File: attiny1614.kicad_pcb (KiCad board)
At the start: 2 copper layers, 14.7 x 18.8 mm, 12 parts, among them J1 Conn_01x07, J2 Conn_01x07, J3 Conn_01x02, J4 UPDI, U1 AP7381-50SA, U2 ATtiny1614-SS

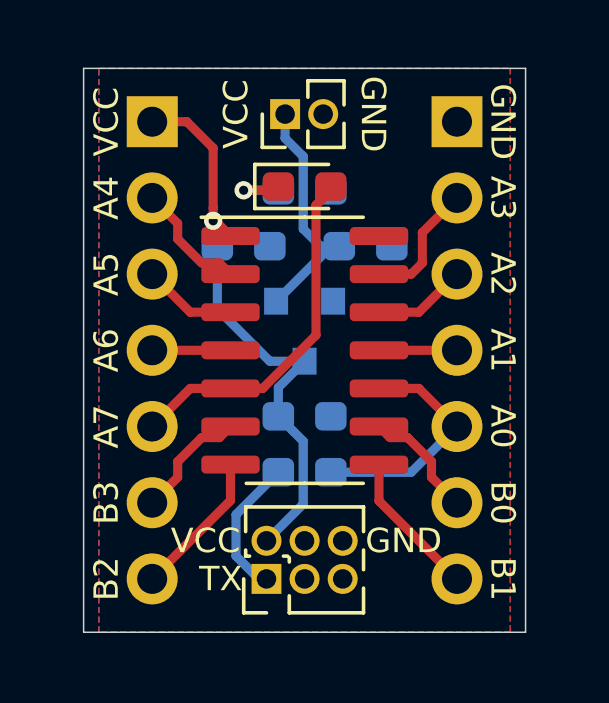
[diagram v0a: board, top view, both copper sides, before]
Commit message: gerbers and layout
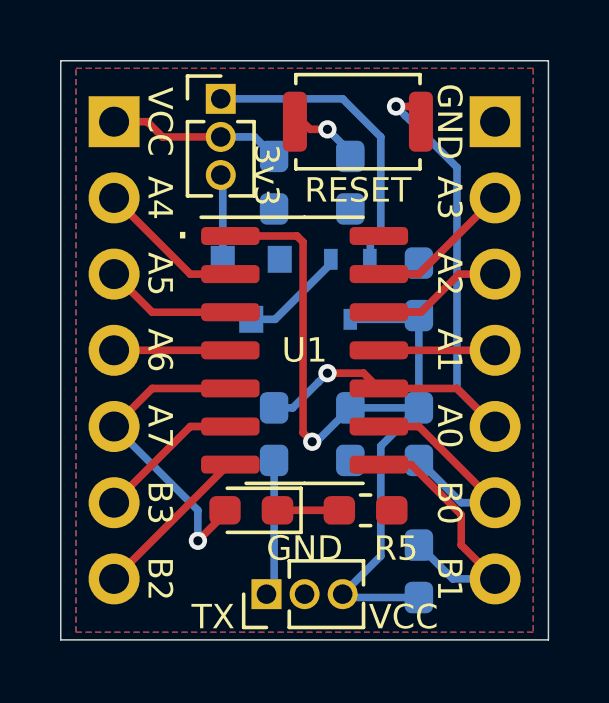
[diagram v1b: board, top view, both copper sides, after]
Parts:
- removed J4: UPDI, Connector_PinHeader_1.27mm:PinHeader_2x03_P1.27mm_Vertical
- added D2: BAT54CW, Package_TO_SOT_SMD:SOT-323_SC-70, B.Cu at (132.1, 87.9)
- added JP1: VCC Select, Connector_PinHeader_1.27mm:PinHeader_1x03_P1.27mm_Vertical, F.Cu at (127.8, 81.5)
- added R3: 10K, Resistor_SMD:R_0603_1608Metric_Pad1.05x0.95mm_HandSolder, B.Cu at (134.4, 97.3)
- added R4: 4.7K, Resistor_SMD:R_0603_1608Metric_Pad1.05x0.95mm_HandSolder, B.Cu at (129.5, 92.7)
- added R5: 2.2K, Resistor_SMD:R_0603_1608Metric_Pad1.05x0.95mm_HandSolder, F.Cu at (132.6, 95.2)
- added SW1: Reset, Button_Switch_SMD:SW_Push_SPST_NO_Alps_SKRK, F.Cu at (132.3, 82.3)
- J1: value Conn_01x07 -> UPDI; footprint Connector_PinHeader_2.54mm:PinHeader_1x07_P2.54mm_Vertical -> Connector_PinHeader_1.27mm:PinHeader_1x03_P1.27mm_Vertical; moved to F.Cu
- J3: value Conn_01x02 -> Conn_01x07; footprint Connector_PinHeader_1.27mm:PinHeader_1x02_P1.27mm_Vertical -> Connector_PinHeader_2.54mm:PinHeader_1x07_P2.54mm_Vertical; moved to B.Cu
- R1: value 4.7K -> 100R
- R2: value 4.7K -> 10K
- U1: value AP7381-50SA -> ATtiny1614-SS; footprint Package_TO_SOT_SMD:SOT-23 -> Package_SO:SOIC-14_3.9x8.7mm_P1.27mm; moved to F.Cu
- U2: value ATtiny1614-SS -> AP7381-33SA; footprint Package_SO:SOIC-14_3.9x8.7mm_P1.27mm -> Package_TO_SOT_SMD:SOT-23; moved to B.Cu
- moved J1 16.2 mm to (129.3, 98.0), turned to 90 degrees
- moved J2 11.4 mm to (124.2, 82.3)
- moved D1 10.9 mm to (128.8, 95.2), turned to 180 degrees
- moved R1 9.77 mm to (132.1, 84.3), turned to 270 degrees
- moved R2 8.98 mm to (134.4, 92.7), turned to 90 degrees
- moved C3 7.20 mm to (132.1, 92.7), turned to 270 degrees
- moved J3 7.00 mm to (136.9, 82.3), turned to 180 degrees
- moved C2 5.69 mm to (134.4, 87.9), turned to 90 degrees
- moved C1 3.71 mm to (129.5, 84.3), turned to 270 degrees
- moved U2 2.70 mm to (128.8, 87.9), turned to 270 degrees
- moved U1 0.63 mm to (130.6, 89.9), turned to 0 degrees
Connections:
- D1 pad 1: Net-(D1-Pad1) -> Net-(D2-Pad1)
- J1 pad 1: VCC -> /TX
- J1 pad 2: /PA4 -> GND
- J1 pad 3: /PA5 -> VCC
- J2 pad 1: GND -> /V_in
- J2 pad 2: /PA3 -> /PA4
- J2 pad 3: /PA2 -> /PA5
- J2 pad 4: /PA1 -> /PA6
- J2 pad 5: /PA0 -> /PA7
- J2 pad 6: /PB0 -> /RXD
- J2 pad 7: /PB1 -> /TXD
- J3 pad 1: /V_in -> GND
- J3 pad 2: GND -> /SCK
- R1 pad 1: /TX -> Net-(R1-Pad1)
- R1 pad 2: /PA0 -> GND
- R2 pad 1: Net-(D1-Pad1) -> /SCL
- R2 pad 2: GND -> VCC
- U1 pad 1: /V_in -> VCC
- U1 pad 2: GND -> /PA4
- U1 pad 3: VCC -> /PA5
- U2 pad 1: VCC -> Net-(JP1-Pad3)
- U2 pad 2: /PA4 -> GND
- U2 pad 3: /PA5 -> Net-(D1-Pad1)
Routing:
- net /PA0: track 7.96 -> 21.6 mm, vias 0 -> 2
- net Net-(D1-Pad2): track 0.00 -> 10.1 mm
- net /SCA: track 0.00 -> 9.05 mm
- net VCC: track 19.4 -> 28.4 mm
- net /SCL: track 0.00 -> 8.05 mm
- net /TXD: track 0.00 -> 5.45 mm
- net /SCK: track 0.00 -> 4.93 mm
- net /RXD: track 0.00 -> 4.93 mm
- net /PB2: track 4.89 -> 0.00 mm
- net /PB1: track 4.89 -> 0.00 mm
- net /MISO: track 0.00 -> 4.40 mm
- net /PA3: track 4.25 -> 0.00 mm
- net /PB3: track 3.97 -> 0.00 mm
- net /PB0: track 3.96 -> 0.00 mm
- net /MOSI: track 0.00 -> 3.88 mm
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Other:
- board size 14.7 x 18.8 mm -> 16.3 x 19.3 mm
- board text added: "."
- board text added: "3v3"
- board text added: "ATtiny1614 v1.2"
- board text added: "RESET"
- board text removed: "ATtiny1614 v1.0"
